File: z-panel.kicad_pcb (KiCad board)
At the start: 2 copper layers, 80 x 80 mm, 27 parts, among them J1 MOLEX_FFC-14, J2 PC104PTH, J3 PC104PTH, J4 PC104PTH, J5 PC104PTH, J6 SMA, U100 OPA380, U110 OPA380, U120 OPA380, U130 OPA380

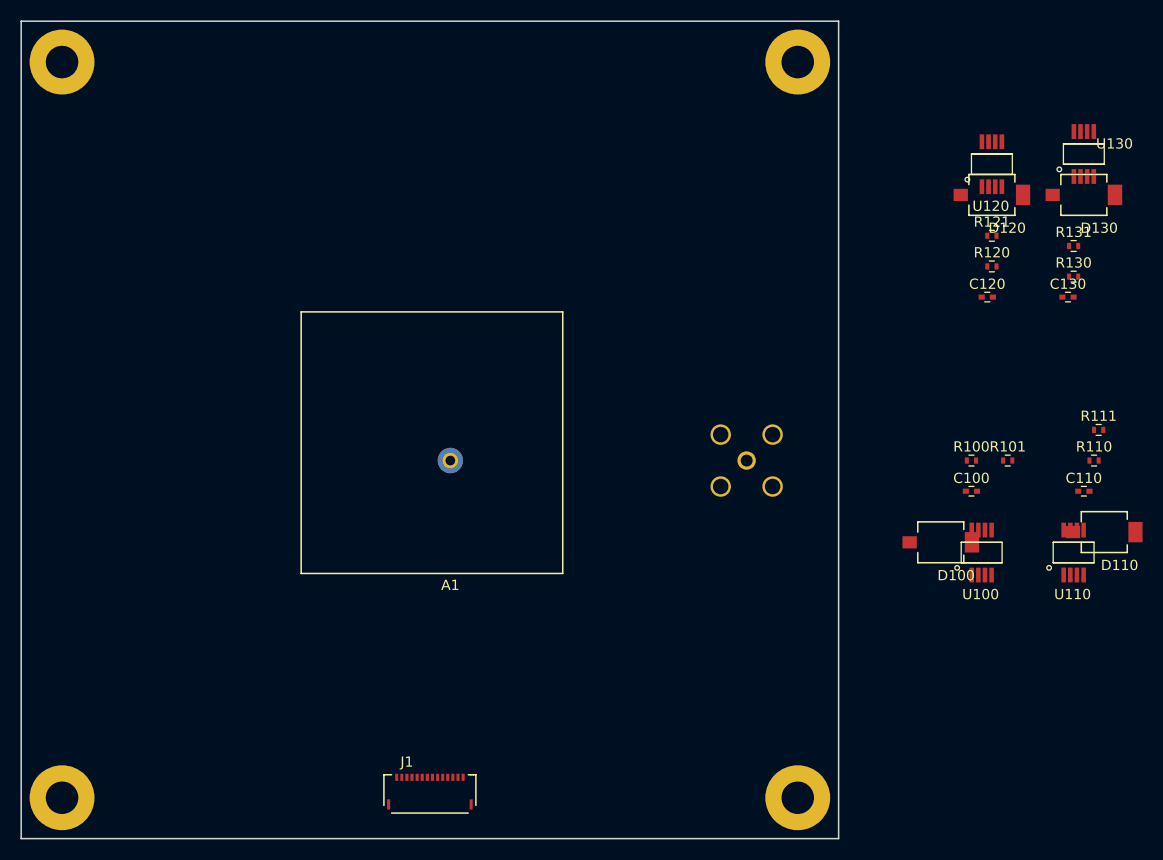
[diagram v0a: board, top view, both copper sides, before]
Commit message: layout complete
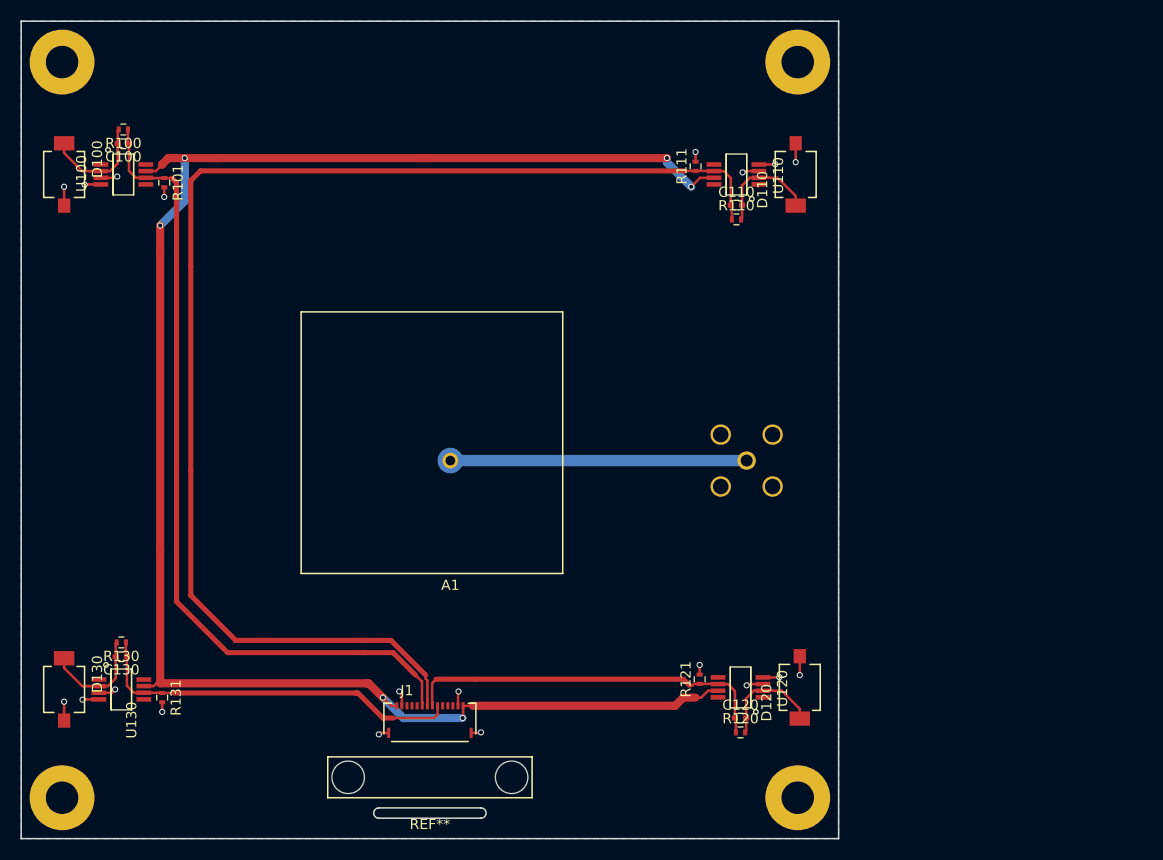
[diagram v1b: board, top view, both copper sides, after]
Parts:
- added REF**: FFC-Fasteners-8mm, SFUSat:FFC-Fasteners-8mm, F.Cu at (150.0, 134.0)
- moved D130 110.9 mm to (114.2, 125.4), turned to 90 degrees
- moved U130 107.8 mm to (119.8, 125.4), turned to 270 degrees
- moved R130 99.8 mm to (119.8, 120.8), turned to 180 degrees
- moved R131 99.6 mm to (123.8, 126.2), turned to 270 degrees
- moved C130 99.1 mm to (119.8, 122.2), turned to 180 degrees
- moved D100 93.0 mm to (114.2, 75.0), turned to 90 degrees
- moved U100 91.8 mm to (120.0, 75.0), turned to 270 degrees
- moved C100 89.7 mm to (120.0, 72.0), turned to 180 degrees
- moved R100 89.1 mm to (120.0, 70.6), turned to 180 degrees
- moved R101 86.9 mm to (124.0, 75.8), turned to 270 degrees
- moved U120 56.8 mm to (180.4, 125.2), turned to 90 degrees
- moved R121 52.0 mm to (176.4, 124.4), turned to 90 degrees
- moved R120 51.8 mm to (180.4, 129.6)
- moved D120 51.7 mm to (186.2, 125.2), turned to 270 degrees
- moved U110 49.6 mm to (180.0, 75.0), turned to 90 degrees
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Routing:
- net /3V3: track 0.00 -> 171.5 mm, vias 0 -> 6
- net /D2: track 0.00 -> 127.5 mm
- net /D1: track 0.00 -> 79.9 mm
- net /D4: track 0.00 -> 37.0 mm
- net /D3: track 0.00 -> 36.7 mm
- net GND: track 0.00 -> 29.3 mm, vias 0 -> 20
- net Net-(A1-Pad1): track 0.00 -> 29.0 mm
- net Net-(C110-Pad2): track 0.00 -> 10.6 mm
- net Net-(C130-Pad2): track 0.00 -> 10.6 mm
- net Net-(C100-Pad2): track 0.00 -> 10.6 mm
- net Net-(C120-Pad2): track 0.00 -> 10.6 mm
- added copper zone on B.Cu, net GND
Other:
- outline, holes or cut-outs redrawn
- net class Long added: clearance 0.2, trace_width 0.25, via_dia 0.6, via_drill 0.4
- net class RF added: clearance 0.2, trace_width 1.11538, via_dia 0.6, via_drill 0.4
